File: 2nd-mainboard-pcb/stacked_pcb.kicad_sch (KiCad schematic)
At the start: 16 parts, among them J12 Steckverbinder_Male_Fans, J13 Steckverbinder_Female_Leistung, J14 Steckverbinder_Male_Leistung, J15 Steckverbinder_Female_Motoren

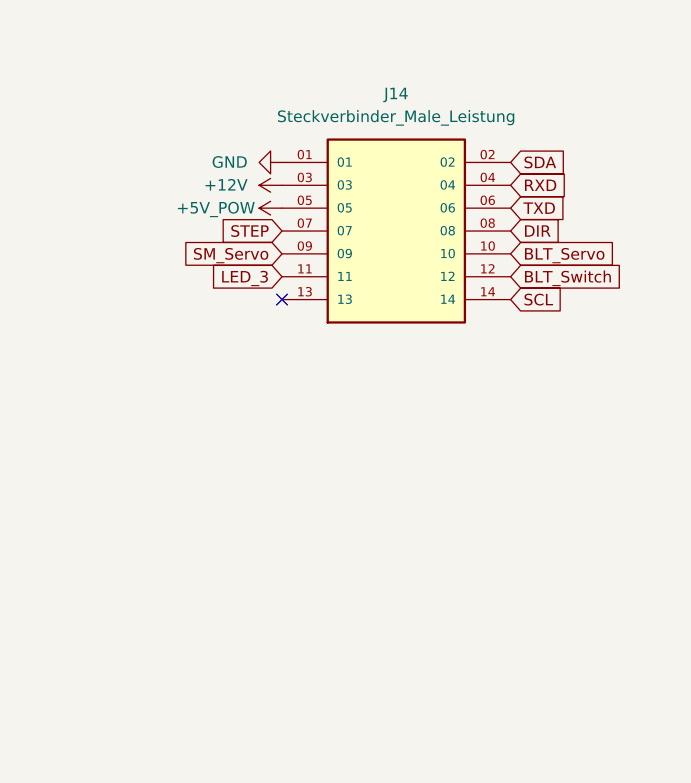
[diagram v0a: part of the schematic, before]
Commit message: cad files gebastelt
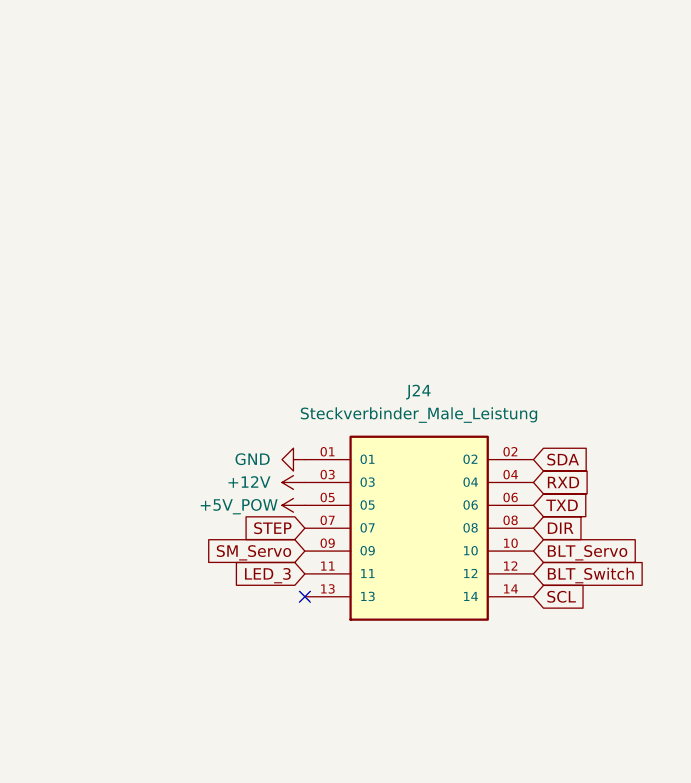
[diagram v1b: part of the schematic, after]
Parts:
- removed J14: Steckverbinder_Male_Leistung, Imported_Component_Footprints:SAMTEC_TSM-107-04-L-DV, symbol Imported_Component_Symbols:TSM-107-04-L-DV
- added J24: Steckverbinder_Male_Leistung, Imported_Component_Footprints:SAMTEC_HW-07-08-L-D-250-SM, symbol Imported_Component_Symbols:HW-07-08-L-D-250-SM
- H1, H2, H3, H4: footprint MountingHole:MountingHole_2.2mm_M2_Pad_TopBottom -> Imported_Component_Footprints:MountingHole_2.7mm_M2.5_ISO7380_Pad_TopBottom_7mm
- H10, H11, H12, H9: footprint MountingHole:MountingHole_2.2mm_M2_Pad_TopBottom -> MountingHole:MountingHole_2.7mm_M2.5_ISO7380_Pad_TopBottom
- H5, H6, H7, H8: footprint MountingHole:MountingHole_2.2mm_M2_Pad_TopBottom -> Imported_Component_Footprints:MountingHole_2.7mm_M2.5_ISO7380_Pad_TopBottom_111mm
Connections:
- net +12V: now also J24.03
- net +5V_POW: now also J24.05
- net BLT_Servo: now also J24.10
- net BLT_Switch: now also J24.12
- net DIR: now also J24.08
- net GND: now also J24.01
- net LED_3: now also J24.11
- net RXD: now also J24.04
- net SCL: now also J24.14
- net SDA: now also J24.02
- net SM_Servo: now also J24.09
- net STEP: now also J24.07
- net TXD: now also J24.06

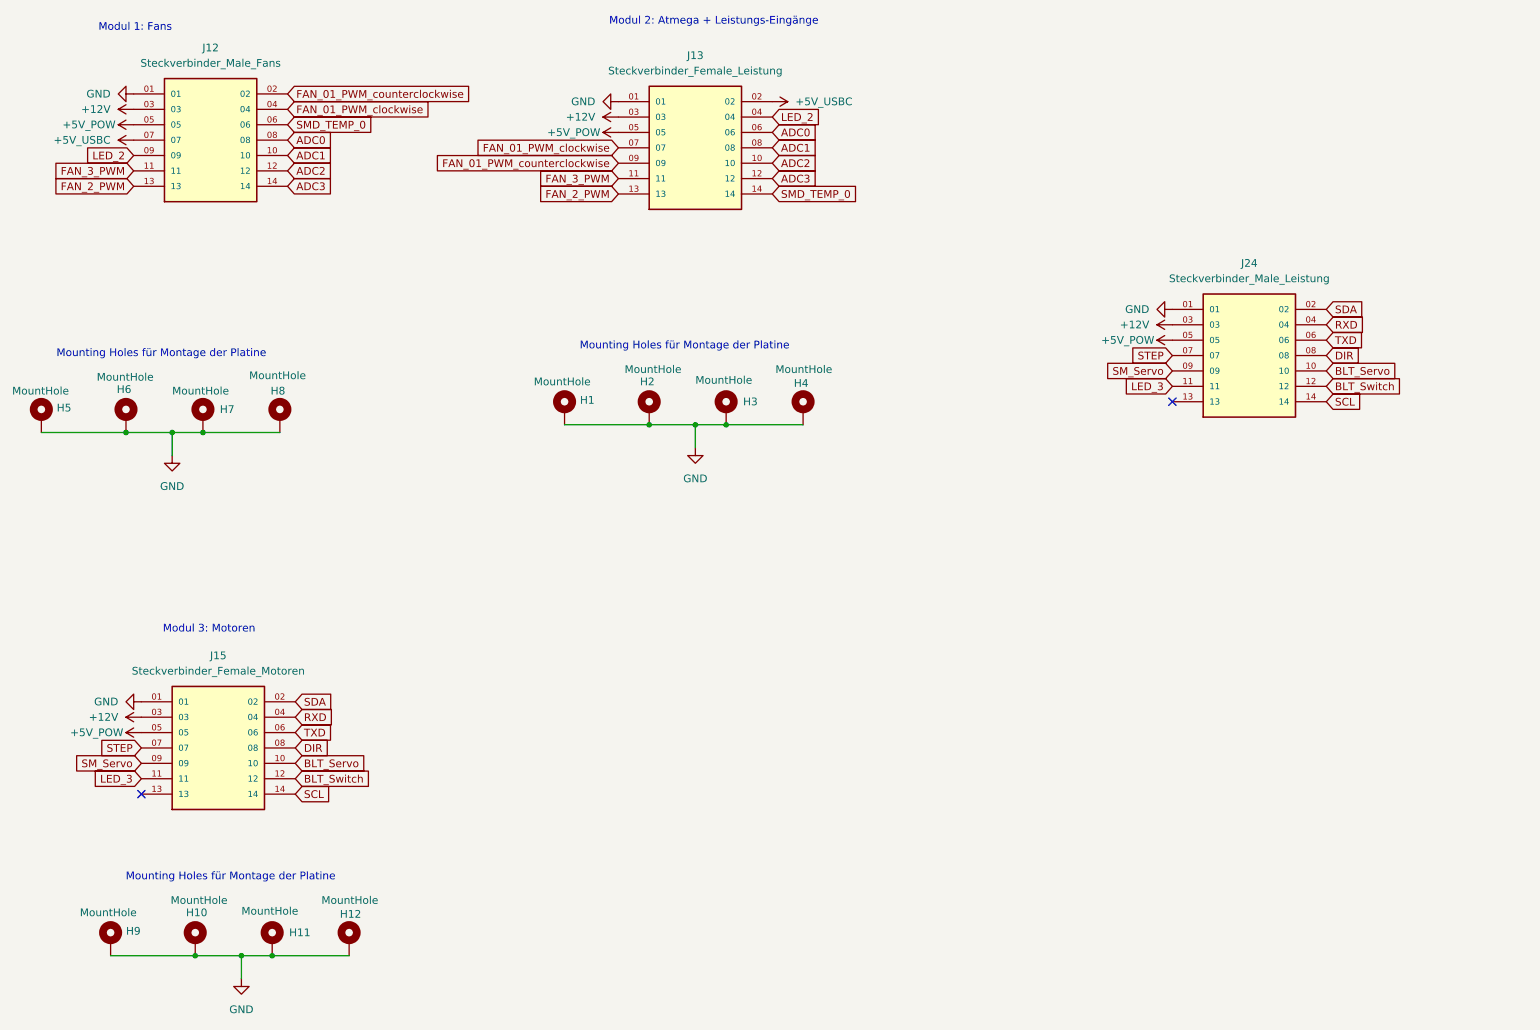
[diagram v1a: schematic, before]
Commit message: stacked pcb reworked
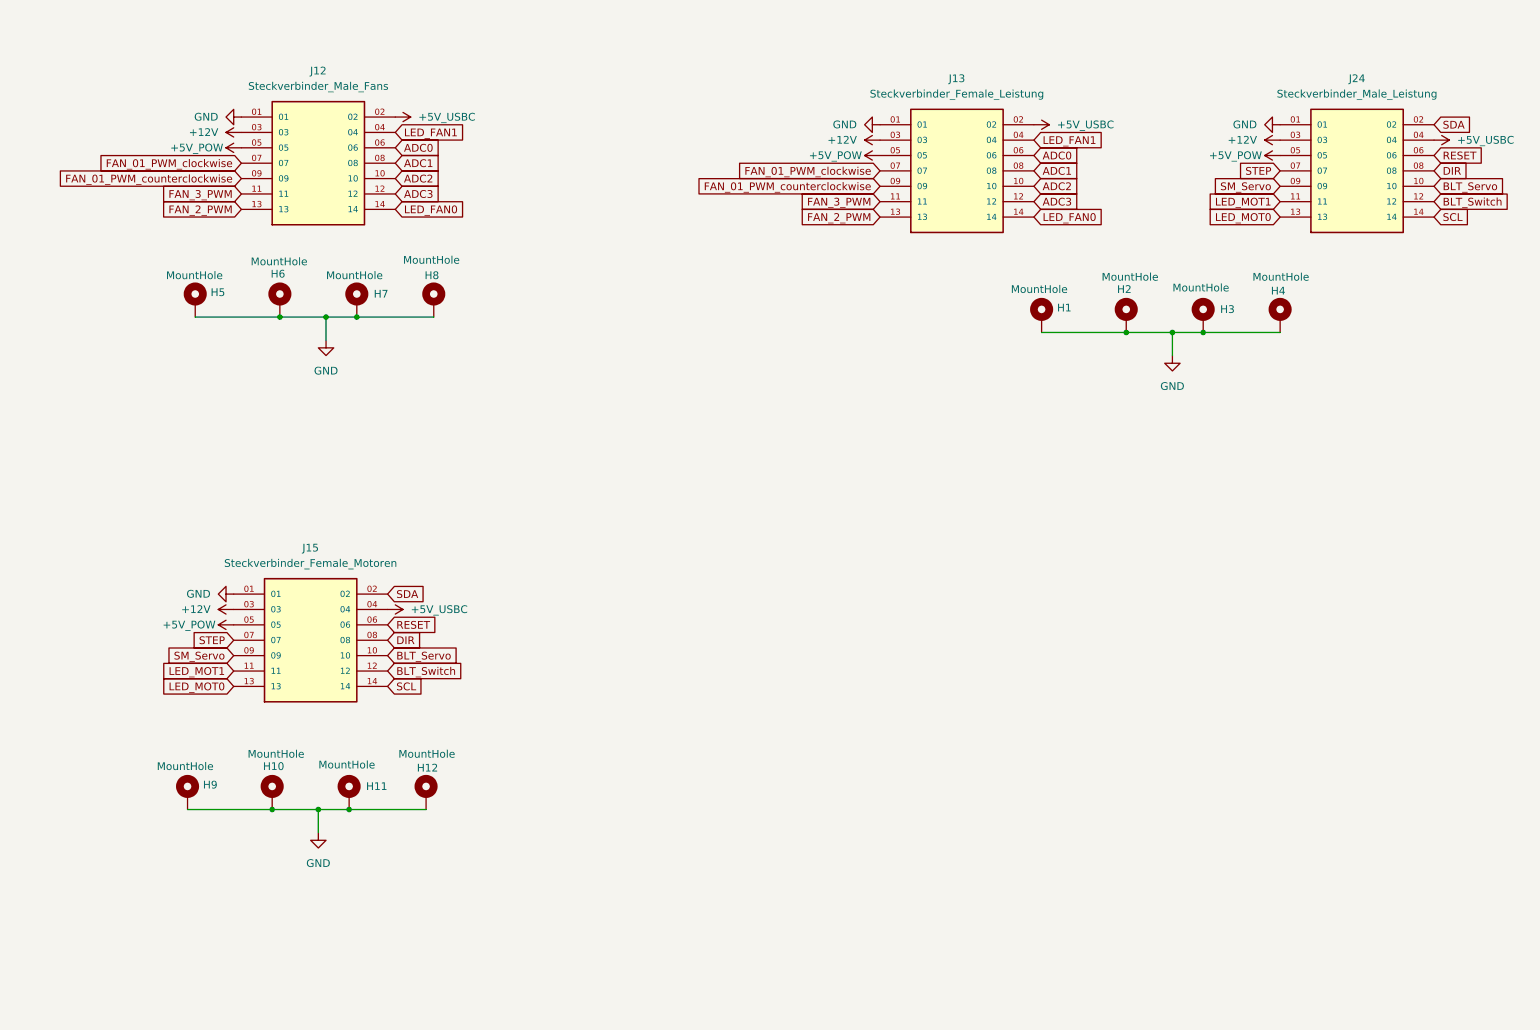
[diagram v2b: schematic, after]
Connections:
- net RXD is gone; now on net +5V_USBC: J15.04, J24.04
- net +5V_USBC: now also J12.02; no longer J12.07
- net ADC0: now also J12.06; no longer J12.08
- net ADC1: now also J12.08; no longer J12.10
- net ADC2: now also J12.10; no longer J12.12
- net ADC3: now also J12.12; no longer J12.14
- net FAN_01_PWM_clockwise: now also J12.07; no longer J12.04
- net FAN_01_PWM_counterclockwise: now also J12.09; no longer J12.02
- net LED_MOT0: now reaches J24.13
- net LED_MOT0: now also J15.13
- net LED_2 renamed LED_FAN1
- net LED_FAN1: now also J12.04; no longer J12.09
- net LED_3 renamed LED_MOT1
- net SMD_TEMP_0 renamed LED_FAN0
- net LED_FAN0: now also J12.14; no longer J12.06
- net TXD renamed RESET
- no-connect marks 2 -> 0
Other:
- note removed: "Modul 1: Fans"
- note removed: "Modul 2: Atmega + Leistungs-Eingänge"
- note removed: "Modul 3: Motoren"
- note removed: "Mounting Holes für Montage der Platine"
- moved on the sheet: H1, H10, H11, H12, H2, H3, H4, H5, H6, H7, H8, H9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
